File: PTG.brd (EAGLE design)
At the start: 105.4 x 82.5 mm, 95 parts, among them IC1 TPS62120, IC2 PIC32MK1024MCF064-I_PT, IC3 LT1762EMS8-5PBF, IC4 TPS561208DDCR, IC5 LT1762EMS8-5PBF, J1 STX-3100-5N, J2 RCJ-01X_PHONO_SINGLE, U4 PCM1748E/2K, X1 22-23-2041, Y1 EXTERNALCRYSTAL

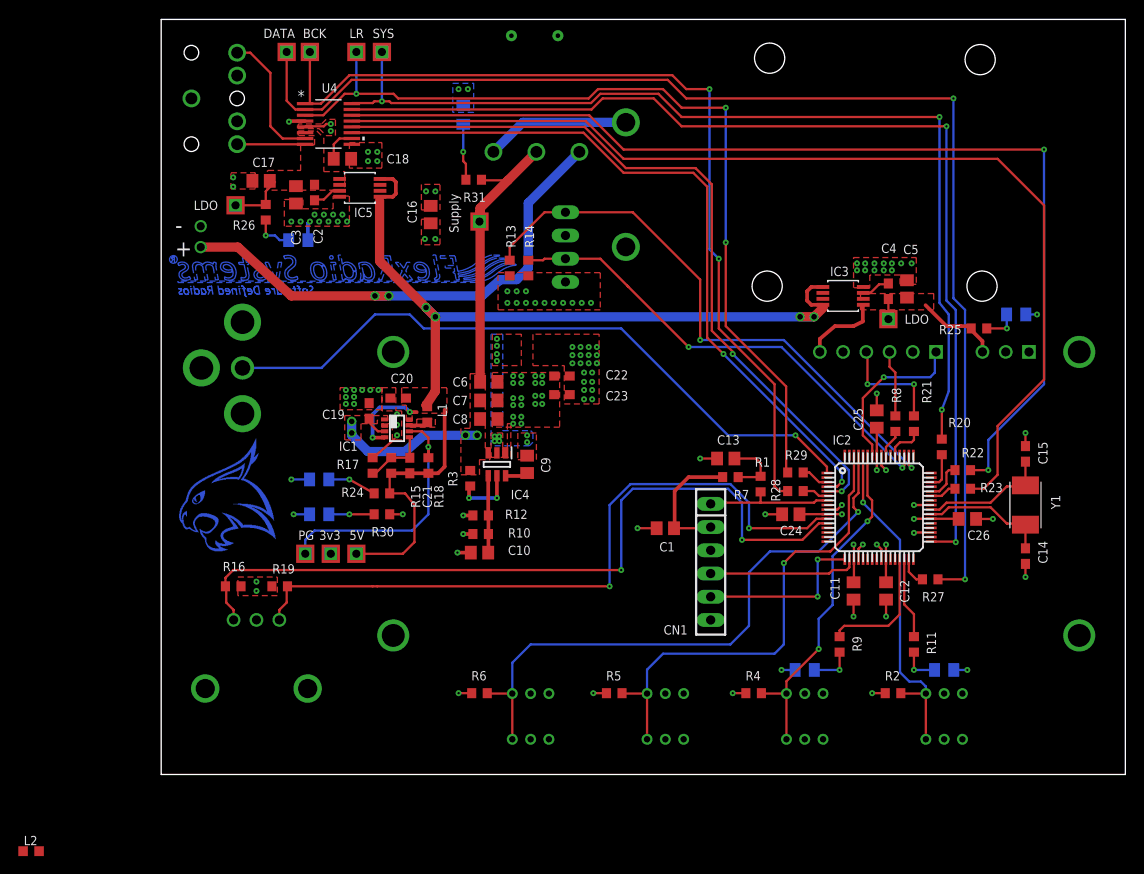
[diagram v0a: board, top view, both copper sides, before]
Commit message: correct file upload
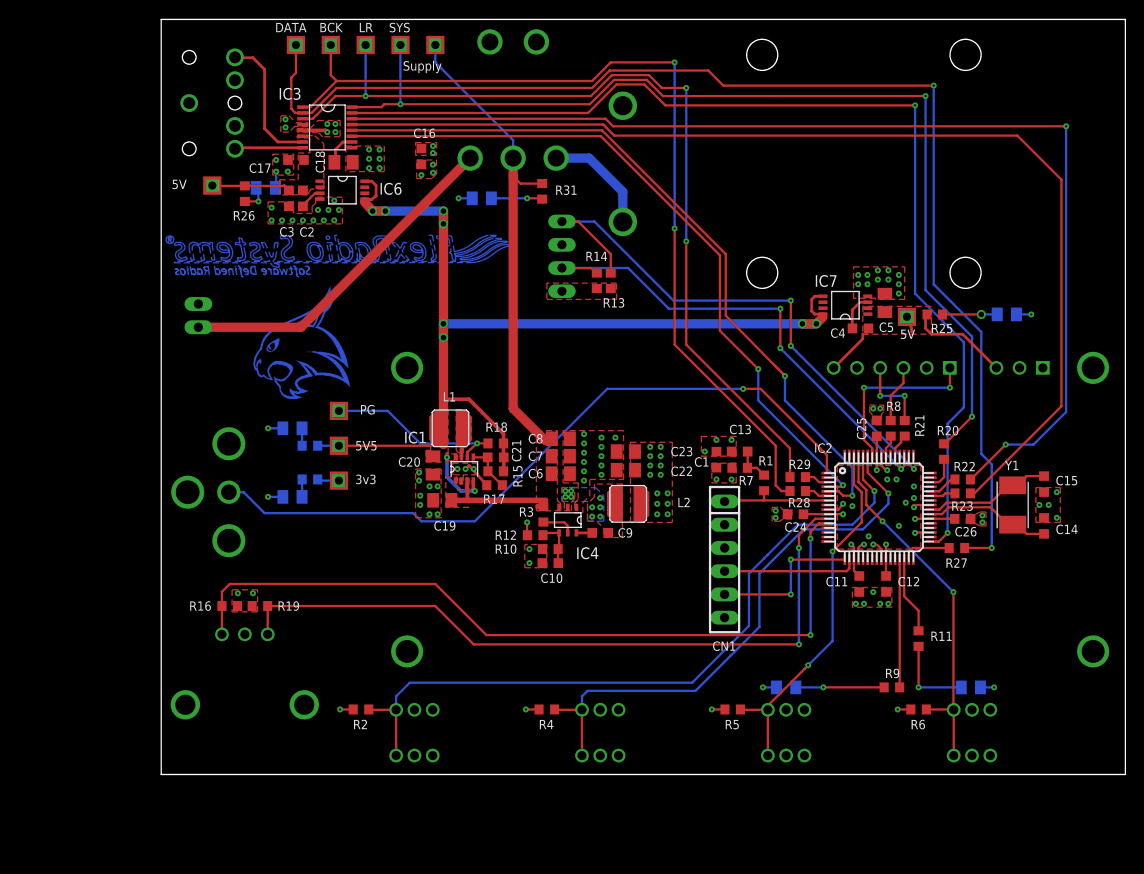
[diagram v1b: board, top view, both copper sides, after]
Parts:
- removed BATT_HOLDER: BATTERY_HOLDER, BattHolder:HOLDER
- removed BUTTON1, BUTTON2, BUTTON3, BUTTON4: BUTTON-DPDT-7MM, button-dpdt-7mm:BUTTON-DPDT-7MM
- removed DIS1: NHD-0216K3Z-FL-GBW-V3, realdisplay:NHD-0216K3Z-FL-GBW-V3
- removed ENC1: ENCODERENCODER, ENCODER_PTG:ENCODER
- removed IC5: LT1762EMS8-5PBF, LDO:MSOP-8_MS
- removed ROCKER_SW: POWERSWITCH, RockerSwitch:ROCKERVIAS
- removed U4: PCM1748E/2K, PCM1748:DBQ16
- added BH1: BATTERY_HOLDER, Batt_Holder:BATTERY_HOLDER
- added D1: NHD-0216K3Z-GBW-V3, NHD-0216K3Z-FL-GBW-V3:NHD-0216K3Z-FL-GBW-V3
- added IC6, IC7: LT1762, LT1762:MS8
- added J3: 22-27-2021-02, con-molex:6410-02
- added SW1: ROCKER_SWITCH, Rocker_Sw:ROCKER_SWITCH
- added SW2: ENCODER, Encoder:EC12E24204A7
- added SW3, SW4, SW5, SW6: MHPS2273N, Button:MHPS2273N
- C1, C10, C11, C12, C13, C16, C17, C24, C25, C26, C9: device rcl:C0805 -> rcl:C0603K
- C14, C15, C2, C21, C4: device rcl:C0603 -> rcl:C0603K
- C18, C5, C6, C7, C8: device rcl:C0805 -> rcl:C0805K
- C19, C20, C22, C23: device rcl:C0603 -> rcl:C0805K
- C3: value 10uF -> 10nF; device rcl:C0805 -> rcl:C0603K
- IC1: device texas:DCN-R-PDSO-G8 -> TPS62120:SOT23(8)
- IC3: value LT1762EMS8-5PBF -> PCM1748; device LDO:MSOP-8_MS -> PCM1748:SSOP
- IC4: value TPS561208DDCR -> TPS561208; device TPS561208DDCR:SOT95P280X110-6N -> TPS561208:SOT6
- J1: value STX-3100-5N -> STX31005NB; device NewSDR:STX-3100-5N -> STX31005NB:STX31005NB
- J2: value RCJ-01X_PHONO_SINGLE -> RCJ-01X; device RCA:RCA_RA_PCB_SINGLE -> RCJ-01X:RCJ-01X
- L1, L2: device NewSDR:C0603K -> VLCF4020Inductor:VLCF4020
- moved L2 75.5 mm to (51.1, 29.6), turned to 270 degrees
- moved IC3 59.3 mm to (18.2, 70.7), turned to 270 degrees
- moved R2 58.2 mm to (21.8, 7.11)
- moved R6 48.0 mm to (82.8, 7.11)
- moved R4 22.7 mm to (42.2, 7.11)
- moved TP5 19.9 mm to (30.0, 79.8)
- moved TP10 16.0 mm to (19.4, 39.8)
- moved J2 15.5 mm to (1.40, 30.9), turned to 180 degrees
- moved R17 13.5 mm to (36.4, 31.6), turned to 0 degrees
- moved R5 13.1 mm to (62.5, 7.11)
- moved C6 12.8 mm to (43.7, 32.9)
- moved C19 12.6 mm to (30.7, 30.0), turned to 180 degrees
- moved C22 12.4 mm to (50.8, 33.3)
- moved TP1 12.0 mm to (19.4, 35.9)
- moved R15 11.4 mm to (36.6, 33.1), turned to 0 degrees
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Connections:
- removed net +5_DAC: C17.1, C2.1, C3.1, IC5.1, IC5.2, R26.2, TP4.1, TP4.TP, U4.6
- removed net 5V_I/O: C20.1, C21.1, IC1.4, IC1.8, IC3.5, IC3.8, IC5.5, IC5.8, L1.2, R15.2, R18.2, R24.2, TP1.1, TP1.TP
- removed net PWR_PIN: ROCKER_SW.1
- removed net SW-B: BATT_HOLDER.+, ROCKER_SW.3
- removed net VOUT_LCD: C4.1, C5.1, DIS1.J1-3, DIS1.J2-6, IC3.1, IC3.2, R25.2, TP3.1, TP3.TP
- new net +5V5: C20.1, C21.1, IC1.4, IC1.8, IC6.5, IC6.8, IC7.5, IC7.8, L1.2, R15.2, R18.2, R24.2, TP1.1, TP1.TP
- new net +5V_DAC: C17.1, C2.1, C3.1, IC3.6, IC6.1, IC6.2, R26.2, TP4.1, TP4.TP
- new net +5V_LCD: C4.1, C5.1, D1.3, D1.9, IC7.1, IC7.2, R25.2, TP3.1, TP3.TP
- new net N$29: BH1.POS, SW1.1
- new net N$30: J3.2, SW1.3
- net !DAC_CS: now also IC3.15; no longer U4.15
- net +3V3: now also IC3.5, SW3.2, SW3.5, SW4.2, SW4.5, SW5.2, SW5.5, SW6.2, SW6.5; no longer BUTTON1.2, BUTTON1.5, BUTTON2.2, BUTTON2.5, BUTTON3.2, BUTTON3.5, BUTTON4.2, BUTTON4.5, U4.5
- net AGND: now also IC3.4, IC3.9, IC6.4; no longer IC5.4, U4.4, U4.9
- net BUTTON1: now also SW3.3, SW3.4; no longer BUTTON1.3, BUTTON1.4
- net BUTTON2: now also SW4.3, SW4.4; no longer BUTTON2.3, BUTTON2.4
- net BUTTON3: now also SW5.3, SW5.4; no longer BUTTON3.3, BUTTON3.4
- net BUTTON4: now also SW6.3, SW6.4; no longer BUTTON4.3, BUTTON4.4
- net DAC_BCK: now also IC3.1; no longer U4.1
- net DAC_DATA: now also IC3.2; no longer U4.2
- net DAC_LRCK: now also IC3.3; no longer U4.3
- net DAC_SPI_CLK: now also IC3.14; no longer U4.14
- net DAC_SPI_DATA: now also IC3.13; no longer U4.13
- net DAC_ZEROH: now also IC3.11; no longer U4.11
- net DAC_ZEROL: now also IC3.12; no longer U4.12
- net DIS_!CS: now also D1.4; no longer DIS1.J2-1
- net DIS_SCK: now also D1.6; no longer DIS1.J2-3
- net DIS_SDI: now also D1.7; no longer DIS1.J2-4
- net ENC_A: now also SW2.A; no longer ENC1.PIN_A
- net ENC_B: now also SW2.B; no longer ENC1.PIN_B
- net GND: now also BH1.NEG, D1.2, D1.8, D1.G1, D1.G2, D1.G3, D1.G4, IC7.4, J2.3, J2.4, J3.1, SW1.G1, SW1.G2, SW2.C, SW2.G1, SW2.G2; no longer BATT_HOLDER.-, DIS1.J1-2, DIS1.J2-5, DIS1.M1, DIS1.M2, DIS1.M3, DIS1.M4, ENC1.PIN_C, IC3.4, J2.1', J2.1''
- net N$19: now also IC3.10; no longer U4.10
- net N$23: now also IC7.3; no longer IC3.3
- net N$9: now also IC6.3; no longer IC5.3
- net SIGNAL_L: now also IC3.7; no longer U4.7
- net SIGNAL_R: now also IC3.8; no longer U4.8
- net SUPPLY: now also SW1.2; no longer ROCKER_SW.2
- net SYS_CLK: now also IC3.16; no longer U4.16
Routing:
- net +5V5: track 0.00 -> 125.4 mm, vias 0 -> 10
- net 5V_I/O: track 120.1 -> 0.00 mm, vias 6 -> 0
- net PWR_PIN: track 55.6 -> 0.00 mm, vias 3 -> 0
- net BUTTON1: track 37.4 -> 79.6 mm
- net N$30: track 0.00 -> 37.4 mm
- net BUTTON4: track 65.8 -> 40.2 mm, vias 1 -> 2
- net BUTTON2: track 37.9 -> 61.4 mm, vias 2 -> 1
- net VOUT_LCD: track 21.0 -> 0.00 mm
- net +5V_LCD: track 0.00 -> 18.3 mm
- net +3V3: track 45.6 -> 27.4 mm, vias 48 -> 32
- net SW-B: track 15.8 -> 0.00 mm
- net SUPPLY: track 50.2 -> 65.5 mm, vias 4 -> 0
- net GND: track 43.3 -> 29.2 mm, vias 73 -> 79
- net BUTTON3: track 52.6 -> 40.4 mm, vias 1 -> 2
- net N$29: track 0.00 -> 12.1 mm
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- added copper zone on layer 1, net +5V5
- added copper zone on layer 1, net +5V_DAC
- added copper zone on layer 1, net +5V_LCD
- removed copper zone on layer 1, net +5_DAC
- removed copper zone on layer 1, net 5V_I/O
- removed copper zone on layer 16, net GND
- removed copper zone on layer 1, net VOUT_LCD
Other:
- board text added: "5V5"
- board text added: "LCD LDO Out"
- board text removed: "+"
- board text removed: "-"
- board text removed: "LDO"
